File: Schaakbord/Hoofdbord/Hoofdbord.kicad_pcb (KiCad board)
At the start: 2 copper layers, 47 parts, among them IC1 SN74LVC2T45DCTRE4, IC2 M24C04-RMN6TP, IC3 MAX6955AAX+, J1 APA102C, J2 5V_Power, J3 Rotary_Encoder, J4 SWD, SW1 SW_Push, SW2 SW_Push, SW3 Boot Modes, U1 STM32F101RDTx, U2 NCP1117-3.3_TO252

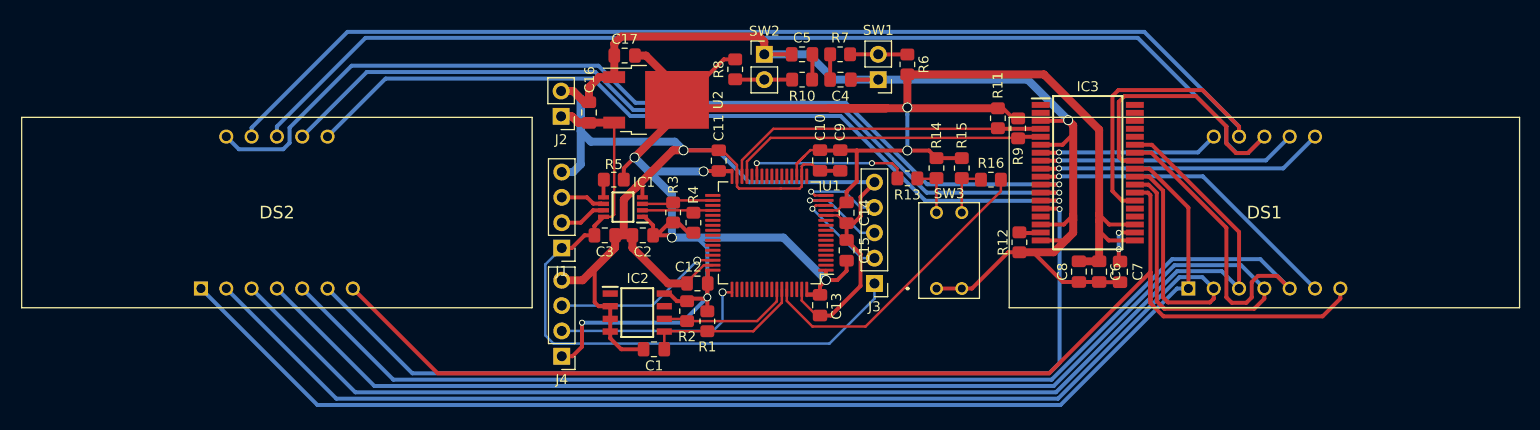
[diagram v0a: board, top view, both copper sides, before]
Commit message: Schematic Update
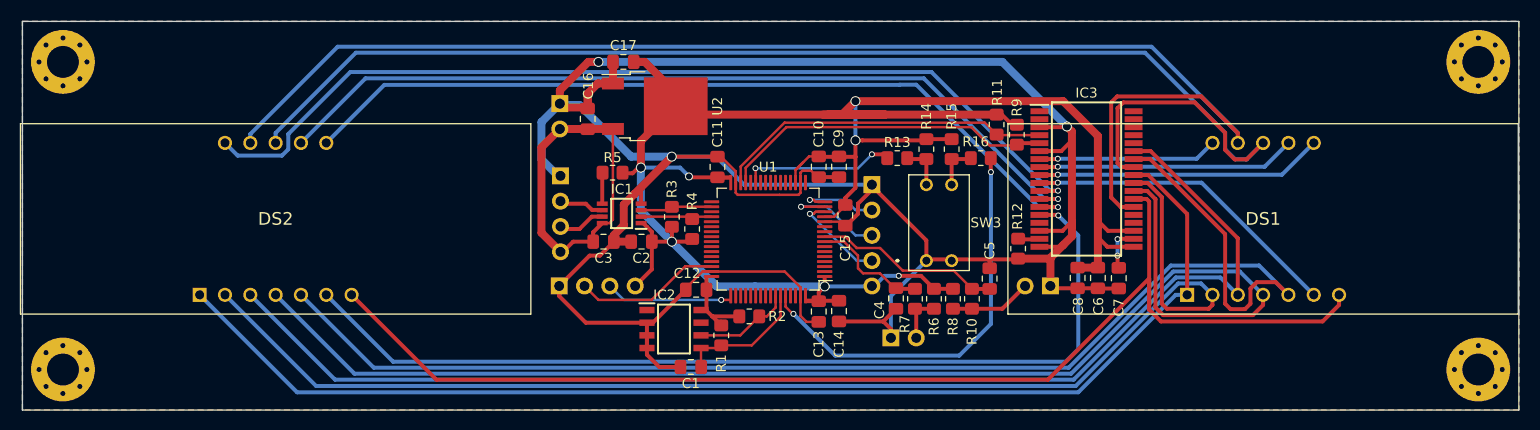
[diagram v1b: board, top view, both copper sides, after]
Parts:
- added ?: MountingHole_3.2mm_M3_Pad_Via, MountingHole:MountingHole_3.2mm_M3_Pad_Via, F.Cu at (94.1, 59.8)
- added ?: MountingHole_3.2mm_M3_Pad_Via, MountingHole:MountingHole_3.2mm_M3_Pad_Via, F.Cu at (236.1, 90.7)
- added ?: MountingHole_3.2mm_M3_Pad_Via, MountingHole:MountingHole_3.2mm_M3_Pad_Via, F.Cu at (94.1, 90.7)
- added ?: MountingHole_3.2mm_M3_Pad_Via, MountingHole:MountingHole_3.2mm_M3_Pad_Via, F.Cu at (236.1, 59.8)
- J1, J2, J3, J4, SW1, SW2: moved to B.Cu
- moved SW2 36.9 mm to (193.2, 82.3), turned to 90 degrees
- moved R8 31.7 mm to (183.4, 83.6)
- moved C5 29.3 mm to (187.1, 81.6), turned to 90 degrees
- moved R10 27.8 mm to (185.3, 83.6), turned to 270 degrees
- moved SW1 25.9 mm to (177.2, 87.5), turned to 270 degrees
- moved R7 25.7 mm to (179.6, 83.6), turned to 270 degrees
- moved R6 23.7 mm to (181.5, 83.6), turned to 90 degrees
- moved C4 22.6 mm to (177.7, 83.5), turned to 270 degrees
- moved J3 9.91 mm to (175.3, 72.1)
- moved C14 9.89 mm to (172.0, 84.8)
- moved J1 7.24 mm to (144.0, 71.2)
- moved J4 7.05 mm to (143.9, 82.3), turned to 270 degrees
- moved R2 6.26 mm to (163.0, 85.3), turned to 180 degrees
- moved C1 4.11 mm to (157.1, 90.4)
- moved IC2 4.04 mm to (155.4, 86.6)
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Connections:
- C4 pad 1: µC -> PC0
- C5 pad 1: µC -> PC1
- J1 pad 1: +5V -> GND
- J1 pad 2: Net-(IC1-Pad7) -> Net-(IC1-Pad6)
- J1 pad 3: Net-(IC1-Pad6) -> Net-(IC1-Pad7)
- J1 pad 4: GND -> +5V
- J2 pad 1: +5V -> GND
- J2 pad 2: GND -> +5V
- J3 pad 1: +5V -> GND
- J3 pad 2: PA0 -> PA2
- J3 pad 4: PA2 -> PA0
- J3 pad 5: GND -> +3V3
- J4 pad 1: +3V3 -> GND
- J4 pad 2: PA14 -> PA13
- J4 pad 3: PA13 -> PA14
- J4 pad 4: GND -> +3V3
- R10 pad 1: µC -> PC1
- R7 pad 1: µC -> PC0
- U1 pad 8: Net-(U1-Pad8) -> PC0
- U1 pad 9: Net-(U1-Pad9) -> PC1
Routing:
- net GND: track 259.3 -> 292.4 mm, vias 2 -> 3
- net +5V: track 68.5 -> 35.6 mm
- net PC1: track 0.00 -> 18.7 mm
- net +3V3: track 246.8 -> 230.1 mm, vias 8 -> 7
- net PC0: track 0.00 -> 11.8 mm
- net BOOT0: track 30.5 -> 41.7 mm, vias 0 -> 2
- net PA14: track 20.4 -> 12.6 mm
- net µC: track 5.09 -> 0.00 mm
- net PB6: track 13.4 -> 9.40 mm
- net PB7: track 16.1 -> 13.3 mm
- net Net-(R10-Pad2): track 5.73 -> 8.19 mm
- net PA13: track 17.1 -> 14.7 mm, vias 1 -> 0
- net Net-(IC1-Pad5): track 1.91 -> 3.51 mm
- net O14: track 129.7 -> 128.2 mm
- net O18: track 128.9 -> 127.3 mm
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- added copper zone on B.Cu, net GND
- added copper zone on F.Cu, net GND
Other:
- board outline added: 150.1 x 39 mm

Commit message: Ontwerp Update
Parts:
- removed the ? at (94.1, 59.8)
- removed the ? at (236.1, 90.7)
- removed the ? at (94.1, 90.7)
- removed the ? at (236.1, 59.8)
- added ?: MountingHole_3.2mm_M3_Pad_Via, MountingHole:MountingHole_3.2mm_M3_Pad_Via, F.Cu at (-71.9, -15.5)
- added ?: MountingHole_3.2mm_M3_Pad_Via, MountingHole:MountingHole_3.2mm_M3_Pad_Via, F.Cu at (70.0, 15.4)
- added ?: MountingHole_3.2mm_M3_Pad_Via, MountingHole:MountingHole_3.2mm_M3_Pad_Via, F.Cu at (-71.9, 15.4)
- added ?: MountingHole_3.2mm_M3_Pad_Via, MountingHole:MountingHole_3.2mm_M3_Pad_Via, F.Cu at (70.0, -15.5)
- moved C17 184.9 mm to (-19.4, -13.6), turned to 270 degrees
- moved C12 182.3 mm to (-8.42, 7.37)
- moved C14 182.3 mm to (5.91, 9.50)
- moved C16 182.3 mm to (-19.3, -9.78)
- moved C3 182.3 mm to (-17.7, 2.54)
- moved C4 182.3 mm to (11.6, 8.23)
- moved C5 182.3 mm to (21.0, 6.24)
- moved C7 182.3 mm to (34.0, 6.20)
- moved C8 182.3 mm to (29.8, 6.18)
- moved C9 182.3 mm to (5.91, -4.97)
- moved DS1 182.3 mm to (40.8, 7.87)
- moved DS2 182.3 mm to (-58.2, 7.87)
- moved J1 182.3 mm to (-22.0, -4.06)
- moved J2 182.3 mm to (-22.1, -11.3)
- moved R10 182.3 mm to (19.2, 8.27)
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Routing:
- net GND: track 292.4 -> 558.0 mm
- net +3V3: track 230.1 -> 241.1 mm, vias 7 -> 8
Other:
- board text added: "Schaakbord M.H."
